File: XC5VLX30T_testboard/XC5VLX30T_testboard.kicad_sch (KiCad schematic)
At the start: 28 parts, among them J1 Conn_01x35_Pin, J10 Conn_01x04_Pin, J11 Conn_01x04_Pin, J12 Conn_01x04_Pin, J13 Conn_01x04_Pin, J14 Conn_01x04_Pin, J2 Conn_01x35_Pin, J3 Conn_01x35_Pin, J4 Conn_01x35_Pin, J5 Conn_01x35_Pin, J6 Conn_01x35_Pin, J7 Conn_01x35_Pin, J8 Conn_01x35_Pin, J9 Conn_01x04_Pin, U1 XC5VLX30T-1FFG665C, X1 SG-5032CCN

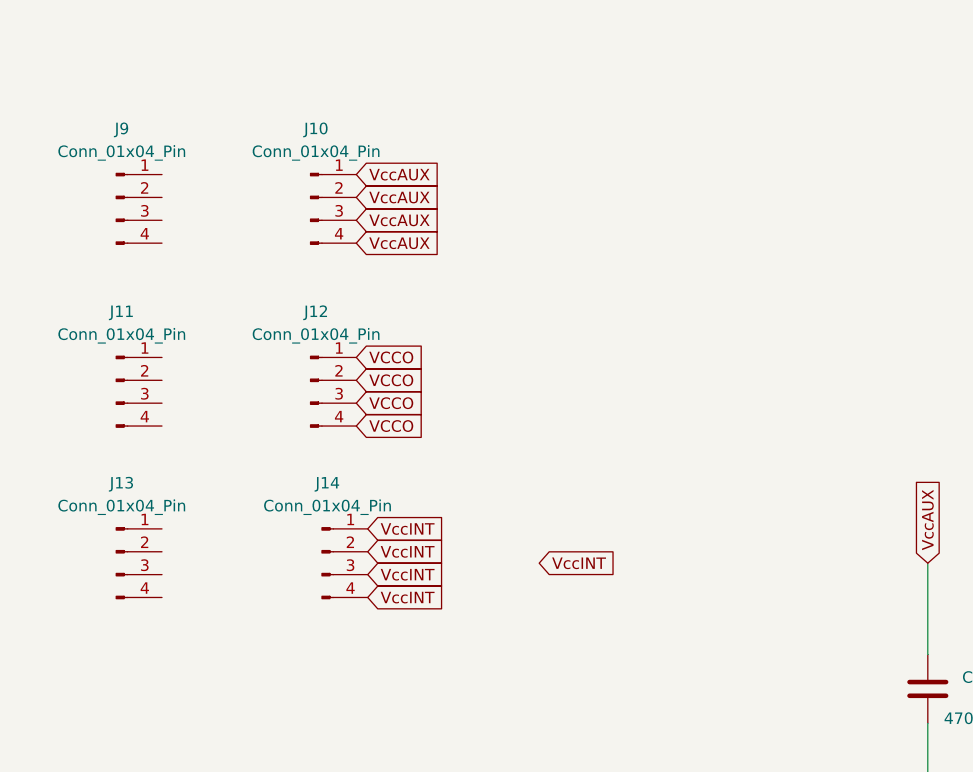
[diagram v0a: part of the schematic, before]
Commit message: more clicking
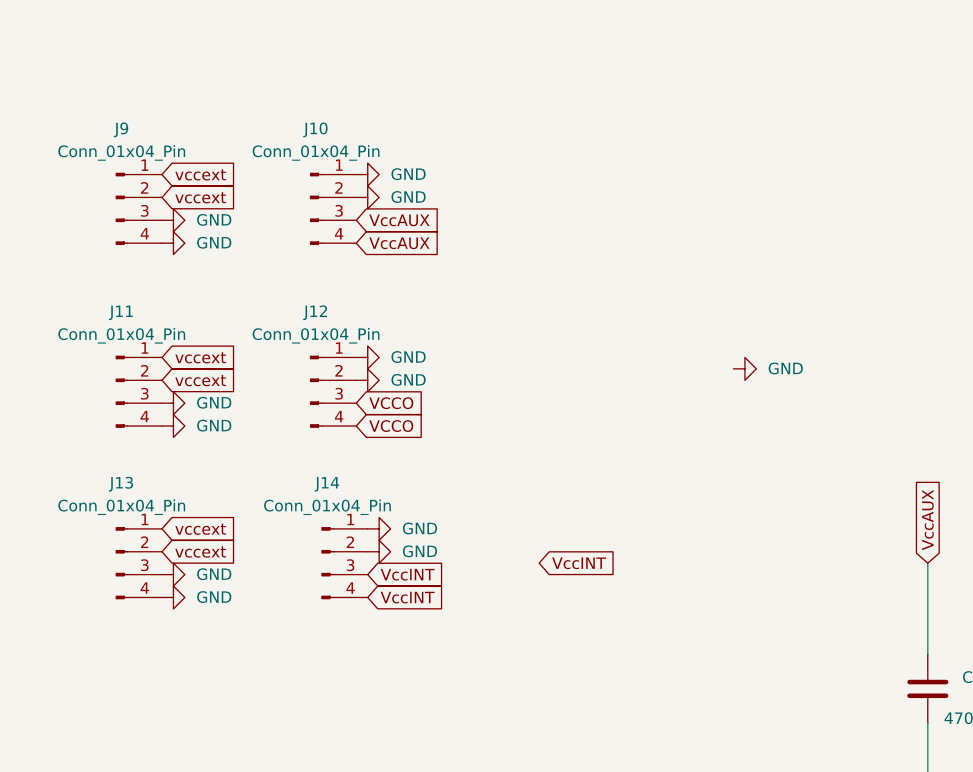
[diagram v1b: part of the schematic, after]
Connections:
- net GND: now also J10.1 (Pin_1), J10.2 (Pin_2), J11.3 (Pin_3), J11.4 (Pin_4), J12.1 (Pin_1), J12.2 (Pin_2), J13.3 (Pin_3), J13.4 (Pin_4), J14.1 (Pin_1), J14.2 (Pin_2), J9.3 (Pin_3), J9.4 (Pin_4)
- net VCCO: no longer J12.1 (Pin_1), J12.2 (Pin_2)
- net VccAUX: no longer J10.1 (Pin_1), J10.2 (Pin_2)
- net VccINT: no longer J14.1 (Pin_1), J14.2 (Pin_2)
- net vccext: now also J11.1 (Pin_1), J11.2 (Pin_2), J13.1 (Pin_1), J13.2 (Pin_2), J9.1 (Pin_1), J9.2 (Pin_2)
